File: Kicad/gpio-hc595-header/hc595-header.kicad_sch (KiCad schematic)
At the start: 8 parts, among them K1 GPIO IN, K2 GPIO OUT, K3 DATA OUT, U1 74HC595, U2 3M-SJ5376

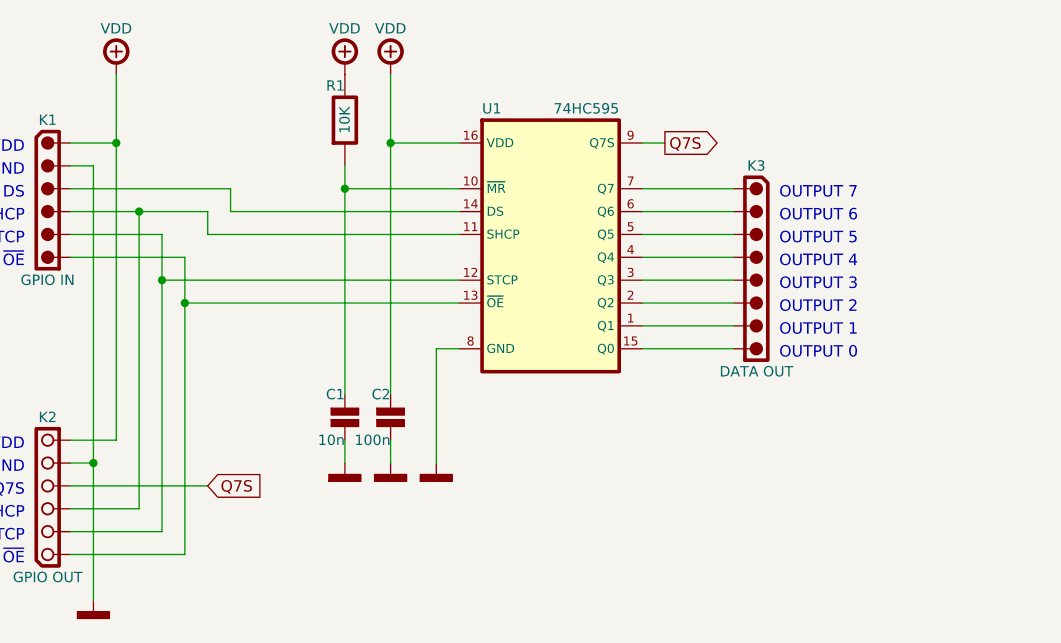
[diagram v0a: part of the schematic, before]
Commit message: Update
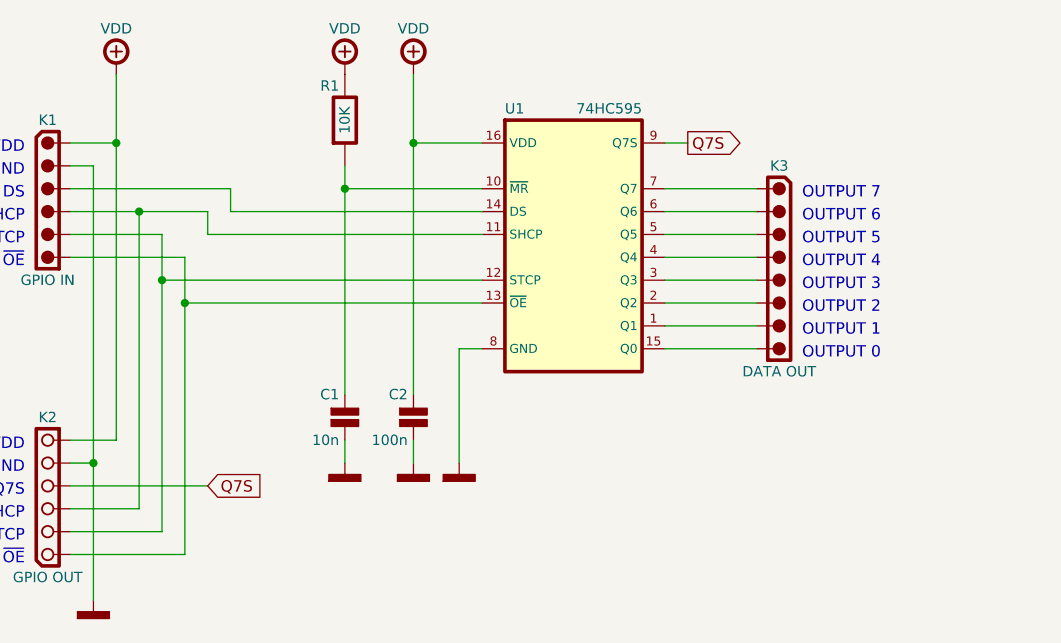
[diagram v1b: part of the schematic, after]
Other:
- moved on the sheet: C2, K3, U1
